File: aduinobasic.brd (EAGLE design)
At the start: 111.1 x 52.4 mm, 85 parts

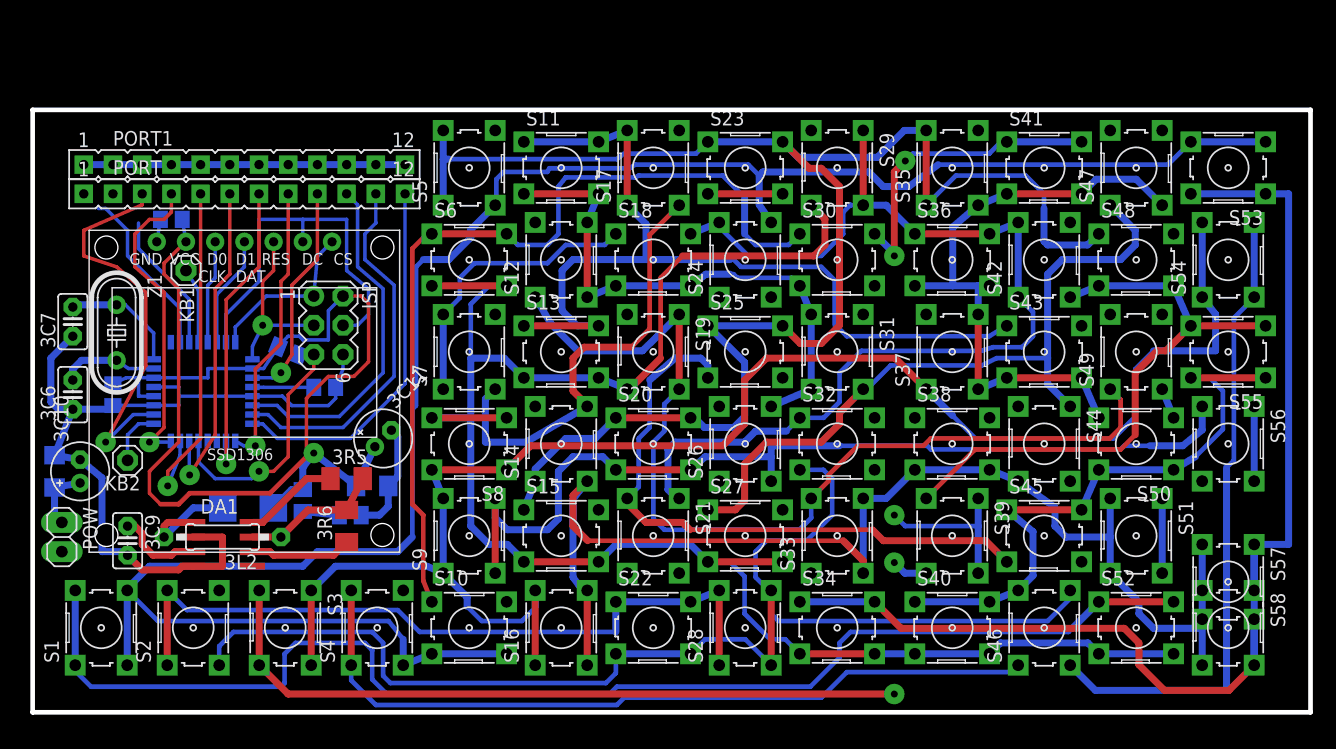
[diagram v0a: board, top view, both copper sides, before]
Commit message: .
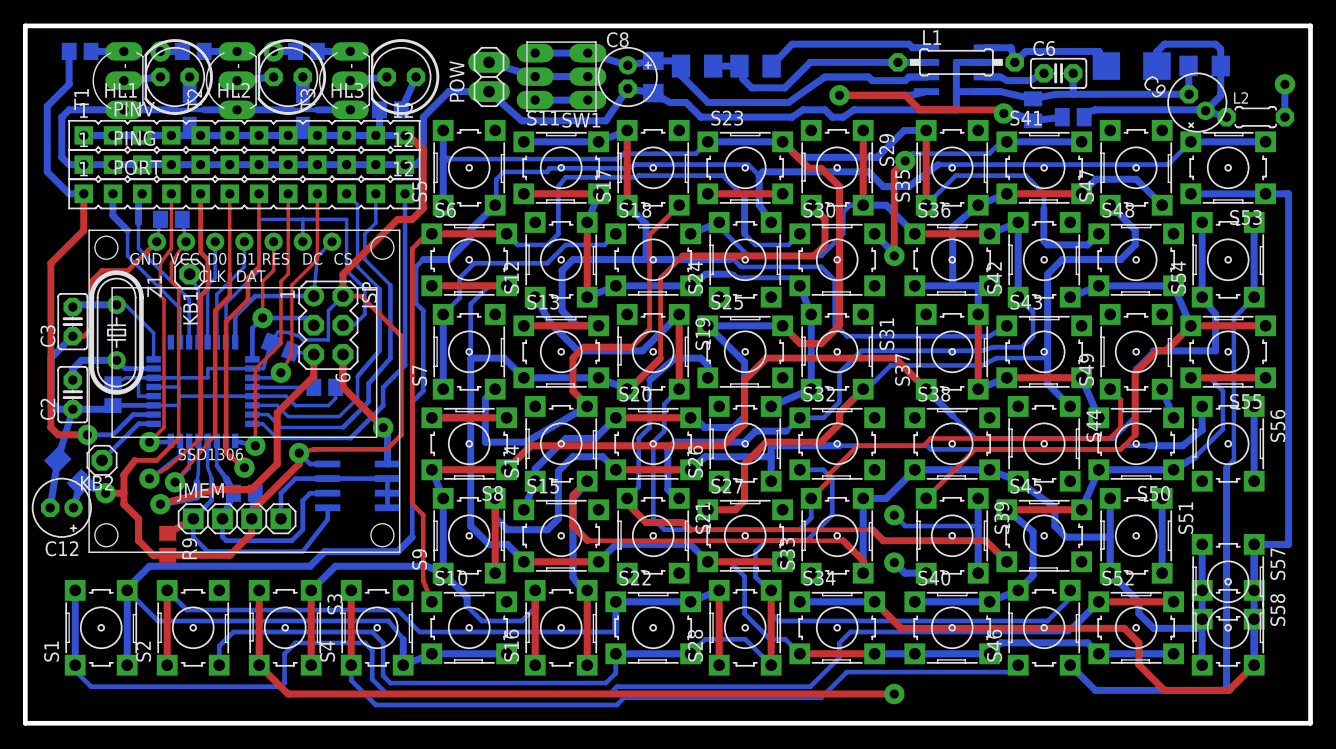
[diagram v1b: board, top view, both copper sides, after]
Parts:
- removed 3C10: 470µ / 10V, HWProgUSB:RCL_E2-5
- removed 3C11: 100µ 16V, HWProgUSB:RCL_E2-5
- removed 3C12: 100n, rcl:C1206
- removed 3C6, 3C7, 3C9: 1n, rcl:C025-025X050
- removed 3C8: 100n, rc-elektronik:C1206
- removed 3L2: 100uh, rcl:0207/10
- removed 3R5: 180, rcl:M1206
- removed 3R6: 1, rcl:M1206
- removed 3R7: 3k, rcl:M0805
- removed 3R8: 1k, rcl:M0805
- removed 3VD2: SS12, diode:SMB
- added C10, C11: 100n, rcl:C1206
- added C12, C9: 100µ 16V, HWProgUSB:RCL_E2-5
- added C4, C5: 100n, rcl:C0805
- added C6: 1n, rcl:C025-025X050
- added C7: 100n, rc-elektronik:C1206
- added C8: 470µ / 10V, HWProgUSB:RCL_E2-5
- added HL1, HL2, HL3: (no value), led:LED5MM
- added IC1: 24LC256SN, microchip:SO-08
- added JMEM: (no value), ArduinoBASIC:1X04
- added L1: 100uh, rcl:0207/10
- added L2: (no value), rcl:0204/5
- added PINV: (no value), ArduinoBASIC:FE12
- added R10: 1, rcl:M1206
- added R11: 180, rcl:M1206
- added R12: 1k, rcl:M0805
- added R13: 3k, rcl:M0805
- added R2, R4, R6, R7, R8, R9: 10k, rcl:R0805
- added R3, R5: 10k, rcl:R1206W
- added SW1: POW, ArduinoBASIC:9077-2
- added T1, T2, T3: (no value), transistor:TO92-ECB
- added VD1: SS12, diode:SMB
- C2, C3: value 100n -> 1n; device rcl:C0805 -> rcl:C025-025X050
- moved DA1 76.0 mm to (106.4, 69.5), flipped to the bottom
- moved POW 54.6 mm to (65.7, 68.9)
- moved C2 21.9 mm to (29.5, 41.3), flipped to the top, turned to 90 degrees
- moved C1 18.4 mm to (51.4, 41.9), turned to 0 degrees
- moved C3 12.3 mm to (29.5, 47.6), flipped to the top, turned to 90 degrees
- moved KB2 2.22 mm to (32.1, 35.6)
- moved R1 0.71 mm to (47.6, 45.4)
- moved KB1 0.45 mm to (39.7, 51.8)
- renumbered PORT1 to PING
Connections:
- new net N$10: SW1.3, SW1.6
- new net N$11: HL1.K, T1.C
- new net N$12: R2.2, T1.B
- new net N$13: HL1.A, R3.1
- new net N$14: HL2.K, T2.C
- new net N$15: R4.2, T2.B
- new net N$16: HL2.A, R5.1
- new net N$17: HL3.K, T3.C
- new net N$18: R6.2, T3.B
- new net N$19: HL3.A, R7.1
- new net N$21: C10.2, C9.+, L2.1, R13.2, VD1.C
- new net N$4: POW.1, SW1.2, SW1.5
- net AREF: now also C1.2; no longer C2.2
- net D14: no longer S33.1
- net D15: no longer S21.2
- net D4: now also PORT.1, R2.1; no longer PORT.3
- net D6: now also PORT.2, R4.1; no longer PORT.1
- net D7: now also PORT.3, R6.1; no longer PORT.2
- net GND: now also C1.1, C10.1, C11.1, C12.-, C3.1, C4.2, C5.2, C6.2, C7.2, C8.-, C9.-, IC1.1, IC1.2, IC1.3, IC1.4, IC1.7, JMEM.4, R12.1, T1.E, T2.E, T3.E; no longer 3C10.-, 3C11.-, 3C12.1, 3C6.1, 3C7.1, 3C8.2, 3C9.2, 3R8.1, C1.2, C3.2
- net N$1: now also C2.2; no longer 3C6.2
- net N$2: now also C3.2; no longer 3C7.2
- net N$3: now also C7.1, C8.+, R10.1, SW1.1, SW1.4; no longer 3C10.+, 3C8.1, 3R6.1, POW.1
- net N$5: now also R11.1; no longer 3R5.1
- net N$6: now also L1.1, R10.2, R11.2; no longer 3L2.1, 3R5.2, 3R6.2
- net N$7: now also R12.2, R13.1; no longer 3R7.1, 3R8.2
- net N$8: now also L1.2, VD1.A; no longer 3L2.2, 3VD2.A
- net N$9: now also C6.1; no longer 3C9.1
- net SCL: now also IC1.5, JMEM.1, R9.1
- net SDA: now also IC1.6, JMEM.2, R8.1
- net U6: no longer S21.4
- net VCC: now also C11.2, C12.+, C4.1, C5.1, IC1.8, JMEM.3, L2.2, PINV.1, PINV.10, PINV.11, PINV.12, PINV.2, PINV.3, PINV.4, PINV.5, PINV.6, PINV.7, PINV.8, PINV.9, R3.2, R5.2, R7.2, R8.2, R9.2; no longer 3C11.+, 3C12.2, 3R7.2, 3VD2.C, C1.1, C3.1
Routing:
- net GND: track 111.6 -> 236.5 mm, vias 0 -> 1
- net VCC: track 105.6 -> 170.5 mm, vias 1 -> 3
- net SCL: track 0.00 -> 26.2 mm
- net N$21: track 0.00 -> 26.0 mm
- net N$7: track 3.19 -> 27.8 mm, vias 0 -> 2
- net N$3: track 13.5 -> 37.3 mm
- net SDA: track 0.00 -> 21.4 mm
- net D4: track 34.2 -> 46.7 mm
- net RESET: track 22.2 -> 32.2 mm
- net N$4: track 0.00 -> 8.78 mm
- net N$6: track 12.2 -> 20.6 mm
- net N$5: track 8.37 -> 14.4 mm
- net N$10: track 0.00 -> 4.58 mm
- net D7: track 12.2 -> 16.8 mm, vias 0 -> 1
- net N$17: track 0.00 -> 3.19 mm
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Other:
- board size 111.1 x 52.4 mm -> 111.8 x 60.6 mm
